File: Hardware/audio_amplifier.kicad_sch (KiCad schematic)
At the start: 8 parts, among them U6 PAM8303DBSC

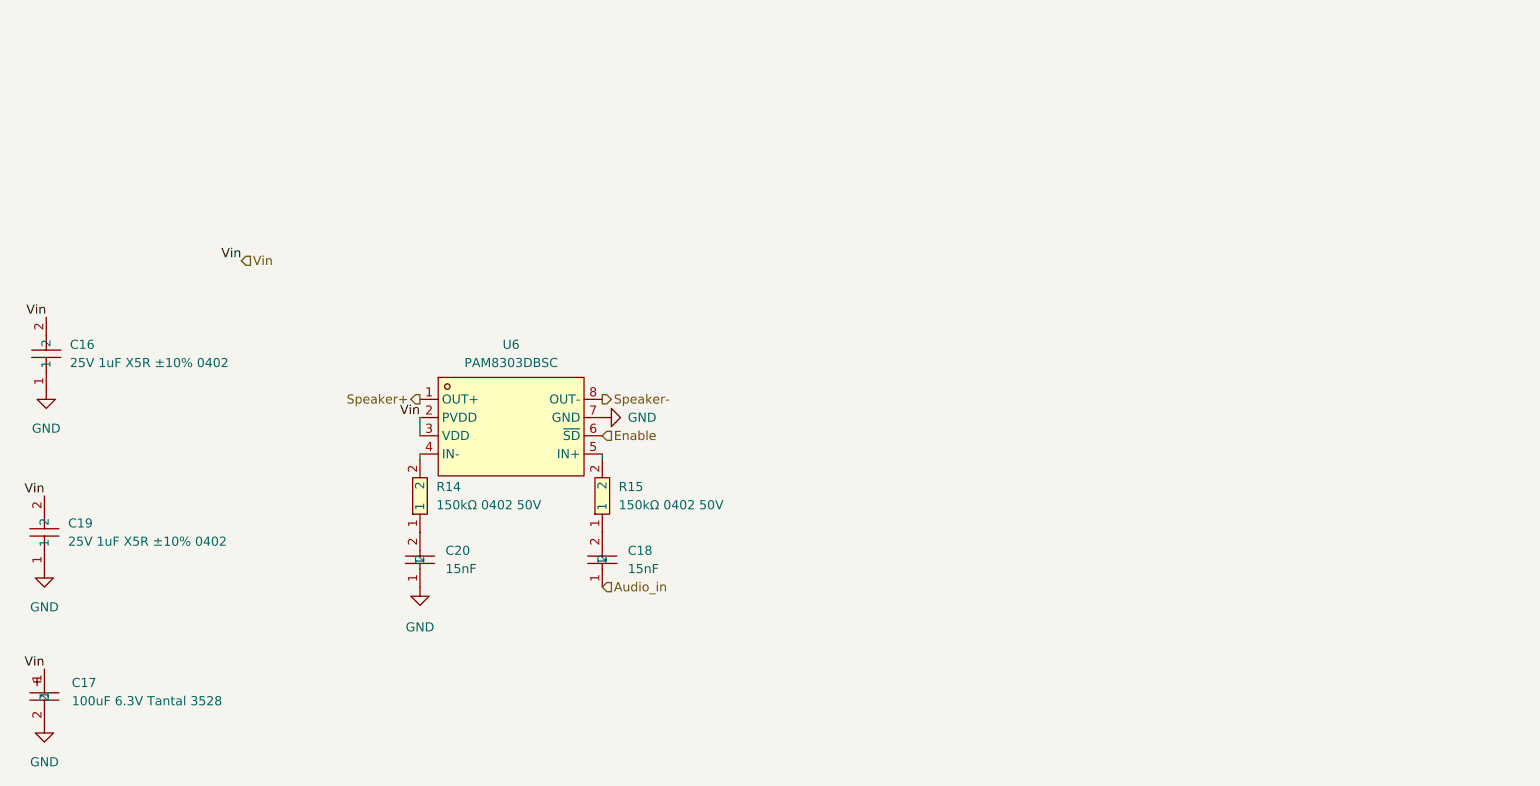
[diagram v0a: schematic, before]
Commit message: PCB V2
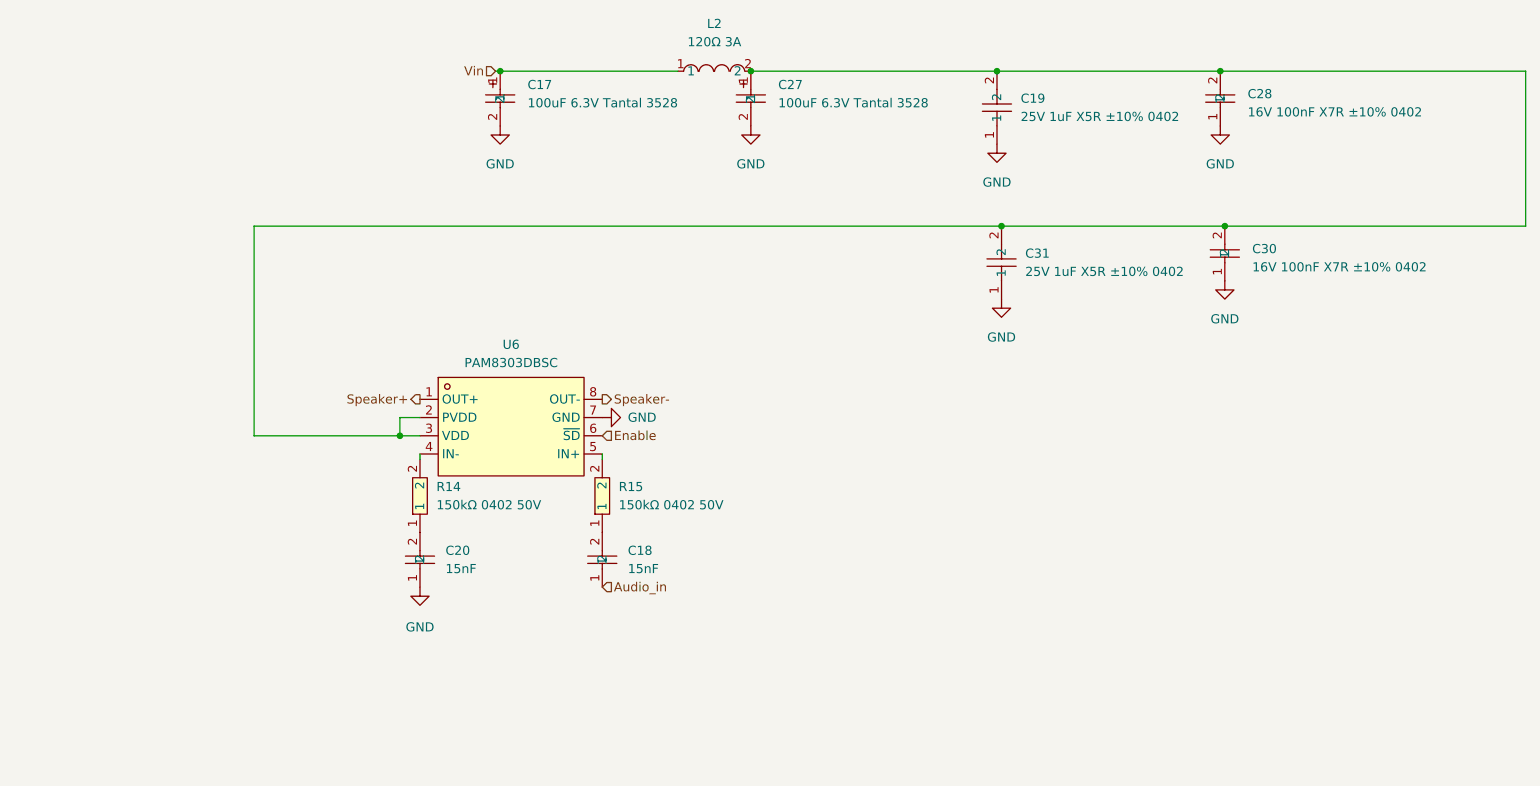
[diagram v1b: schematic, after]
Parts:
- removed C16: 25V 1uF X5R ±10% 0402, easyeda2kicad:C0402, symbol easyeda2kicad:25V 1uF X5R ±10% 0402
- added C27: 100uF 6.3V Tantal 3528, easyeda2kicad:CAP-SMD_L3.5-W2.8, symbol easyeda2kicad:100uF 6.3V Tantal 3528
- added C28, C30: 16V 100nF X7R ±10% 0402, easyeda2kicad:C0402_NEW, symbol easyeda2kicad:16V 100nF X7R ±10% 0402
- added C31: 25V 1uF X5R ±10% 0402, easyeda2kicad:C0402, symbol easyeda2kicad:25V 1uF X5R ±10% 0402
- added L2: 120Ω 3A, easyeda2kicad:L1206, symbol easyeda2kicad:120Ω 3A
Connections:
- net GND: now also C27.2, C28.1, C30.1, C31.1
- net Vin: now also L2.1; no longer C19.2, U6.2 (PVDD), U6.3 (VDD)
- new net: C19.2, C27.1, C28.2, C30.2, C31.2, L2.2, U6.2 (PVDD), U6.3 (VDD)
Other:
- moved on the sheet: C17, C19
